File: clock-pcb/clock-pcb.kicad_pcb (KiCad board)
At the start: 2 copper layers, 66 x 42 mm, 110 parts, among them IC2 MCP23018-E_MJ, J1 Conn_01x03_Pin, J11 Conn_01x06_Socket, J15 Conn_01x02_Socket, J2 oled 2, J3 Led display, J4 Led display 2, J5 Conn_01x07_Socket, J6 Conn_01x07_Socket, J7 SFV25R-2STE1HLF, J8 SFV25R-2STE1HLF, J9 Conn_01x04_Socket, U1 ESP32-C6-MINI-1-N4, U4 TPS2116DRL, U5 MCP73811T-420I-OT, U6 TPS61040DBV, U7 TLV75533PDBV, U8 AT42QT2120-MMHR, Y2 32.768KHz

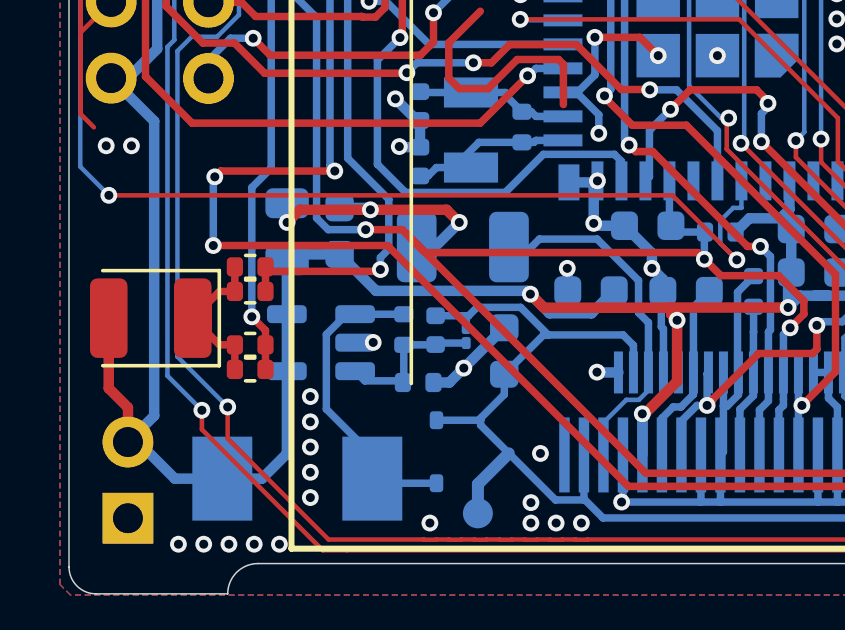
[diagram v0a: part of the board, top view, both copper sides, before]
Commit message: not compiling yet
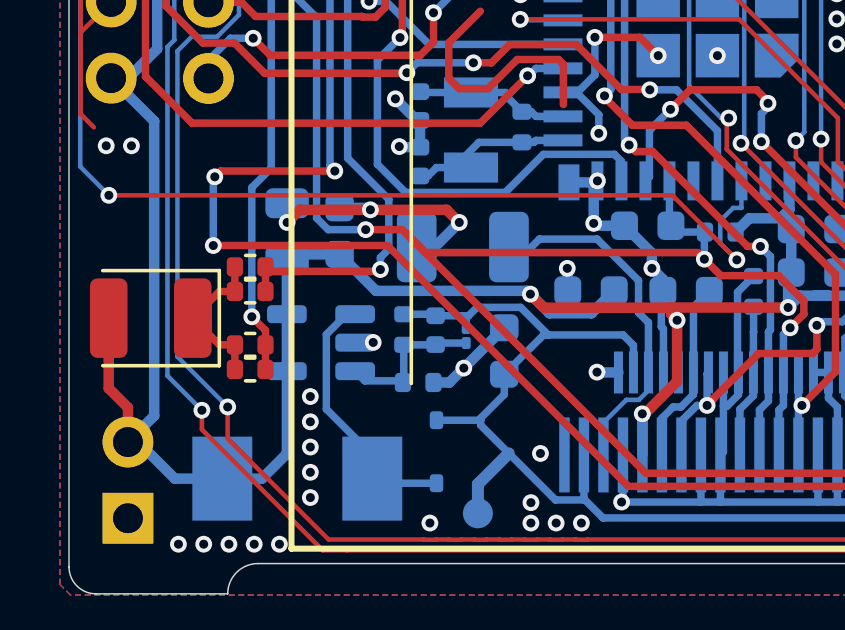
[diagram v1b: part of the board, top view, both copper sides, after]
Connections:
- R27 pad 1: Net-(D3-A) -> 14V_OLED
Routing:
- net Net-(D3-A): track 10.7 -> 9.03 mm
- net 14V_OLED: track 51.7 -> 52.7 mm
